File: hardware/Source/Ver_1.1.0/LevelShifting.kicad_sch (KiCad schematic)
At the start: 42 parts, among them Q1 LN2302LT1G, Q2 LN2302LT1G, Q3 LN2302LT1G, Q4 LN2302LT1G, Q5 LN2302LT1G, Q6 LN2302LT1G

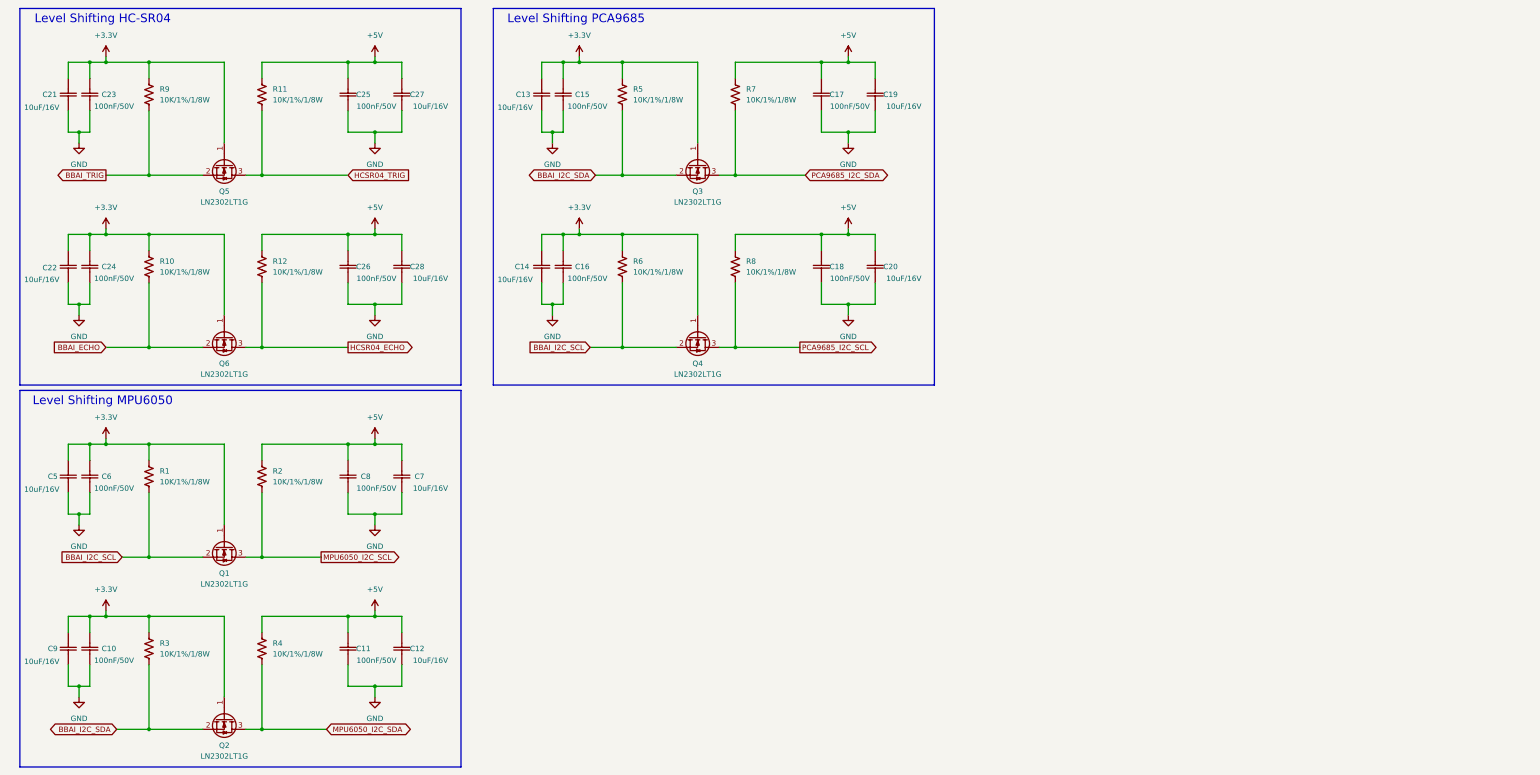
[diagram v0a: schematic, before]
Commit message: update pcb v1.1.0
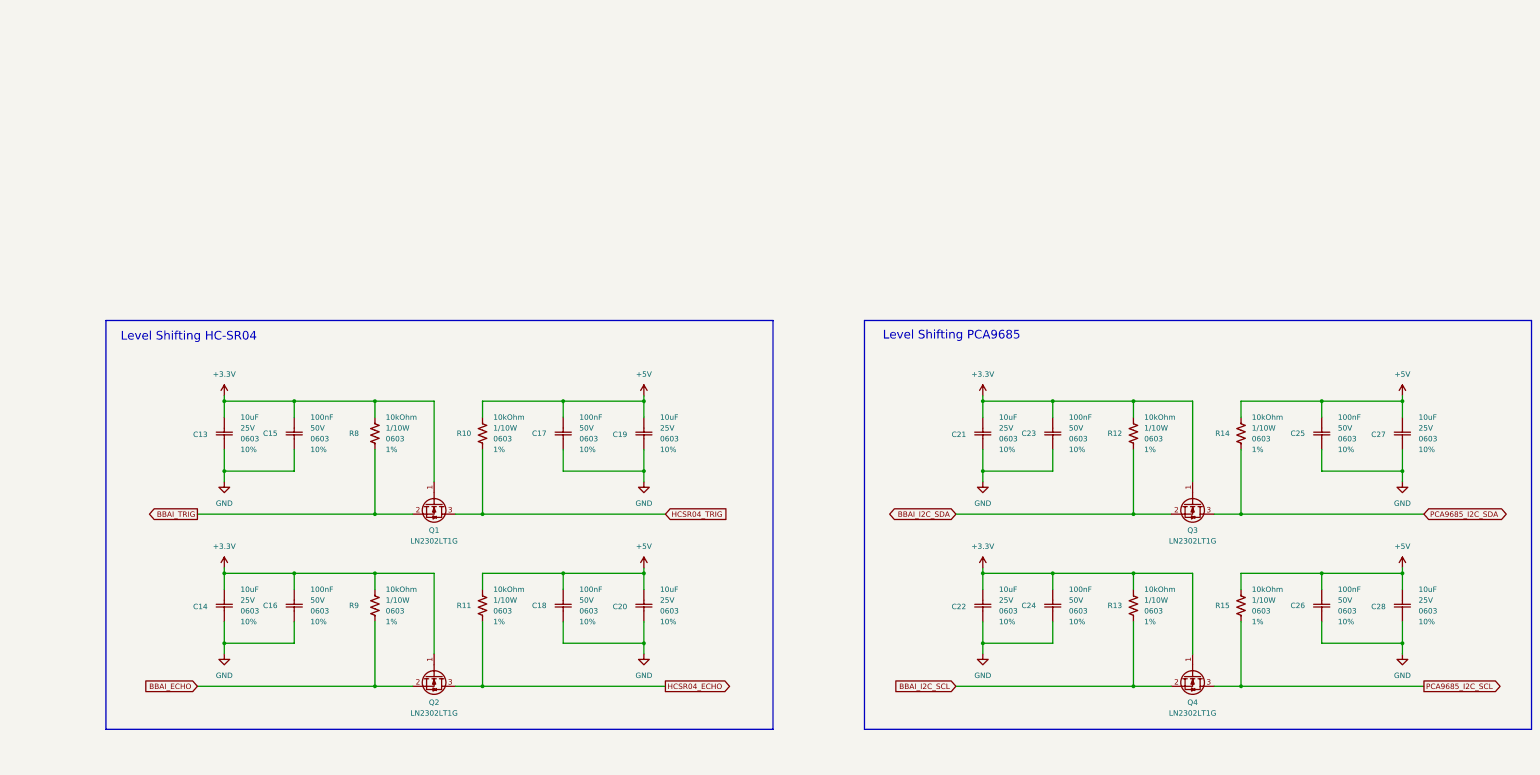
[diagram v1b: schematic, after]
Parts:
- removed C10, C11, C15, C16, C17, C18, C23, C24, C25, C26, C6, C8: 100nF/50V, automative_hexapod:Ceramic_Cap_0805, symbol automative_hexapod:Ceramic_Cap_0805_100nF_50V
- removed C12, C13, C14, C19, C20, C21, C22, C27, C28, C5, C7, C9: 10uF/16V, automative_hexapod:Ceramic_Cap_0805, symbol automative_hexapod:Ceramic_Cap_0805_10uF_16V
- removed Q1, Q6: LN2302LT1G, automative_hexapod:SOT23, symbol automative_hexapod:LN2302LT1G
- removed R1, R10, R11, R12, R2, R3, R4, R5, R6, R7, R8, R9: 10K/1%/1/8W, automative_hexapod:Res_0805, symbol automative_hexapod:Res_10K_0805_1%
- added C13, C14, C19, C20, C21, C22, C27, C28: 10uF, automative_hexapod:Ceramic_Cap_0603, symbol automative_hexapod:Ceramic_Cap_0603_10uF_25V
- added C15, C16, C17, C18, C23, C24, C25, C26: 100nF, automative_hexapod:Ceramic_Cap_0603, symbol automative_hexapod:Ceramic_Cap_0603_100nF_50V
- added R10, R11, R12, R13, R14, R15, R8, R9: 10kOhm, automative_hexapod:Res_0603, symbol automative_hexapod:Res_10K_0603_1%
- Q1: renamed from Q5; Supply Name (none) -> Thegioiic; Supply Part Number (none) -> LN2302LT1G MOSFET Kênh N 20V 2.3A SOT-23-3; Supply URL https://www.thegioiic.com/ln2302lt1g-mosfet-kenh-n-20v-2-3a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 -> https://www.Thegioiic.com/ln2302lt1g-mosfet-kenh-n-20v-2-3a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; Supply name Thegioiic -> (none); Supply part number LN2302LT1G MOSFET Kênh N 20V 2.3A SOT-23-3 -> (none)
- Q2, Q3, Q4: Supply Name (none) -> Thegioiic; Supply Part Number (none) -> LN2302LT1G MOSFET Kênh N 20V 2.3A SOT-23-3; Supply URL https://www.thegioiic.com/ln2302lt1g-mosfet-kenh-n-20v-2-3a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 -> https://www.Thegioiic.com/ln2302lt1g-mosfet-kenh-n-20v-2-3a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; Supply name Thegioiic -> (none); Supply part number LN2302LT1G MOSFET Kênh N 20V 2.3A SOT-23-3 -> (none)
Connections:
- net MPU6050_I2C_SDA is gone; now on net HCSR04_ECHO: Q2.3 (D)
- net +3.3V: now also C13.2, C14.2, C15.2, C16.2, C21.2, C22.2, C23.2, C24.2, R12.2, R13.2, R8.2, R9.2
- net +5V: now also C17.2, C18.2, C19.2, C20.2, C25.2, C26.2, C27.2, C28.2, R10.2, R11.2, R14.2, R15.2
- net BBAI_ECHO: now also Q2.2 (S), R9.1
- net BBAI_I2C_SCL: now also R13.1
- net BBAI_I2C_SDA: now also R12.1; no longer Q2.2 (S)
- net BBAI_TRIG: now also R8.1
- net GND: now also C13.1, C14.1, C15.1, C16.1, C17.1, C18.1, C19.1, C20.1, C21.1, C22.1, C23.1, C24.1, C25.1, C26.1, C27.1, C28.1
- net HCSR04_ECHO: now also R11.1
- net HCSR04_TRIG: now also R10.1
- net PCA9685_I2C_SCL: now also R15.1
- net PCA9685_I2C_SDA: now also R14.1
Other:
- note removed: "Level Shifting MPU6050"
- title: (none) -> LEVEL SHIFTING
- moved on the sheet: Q1
